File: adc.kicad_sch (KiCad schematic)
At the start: 37 parts, among them J5 Conn_01x03_Pin, J8 Conn_01x03_Pin, U21 LTC2299xUP

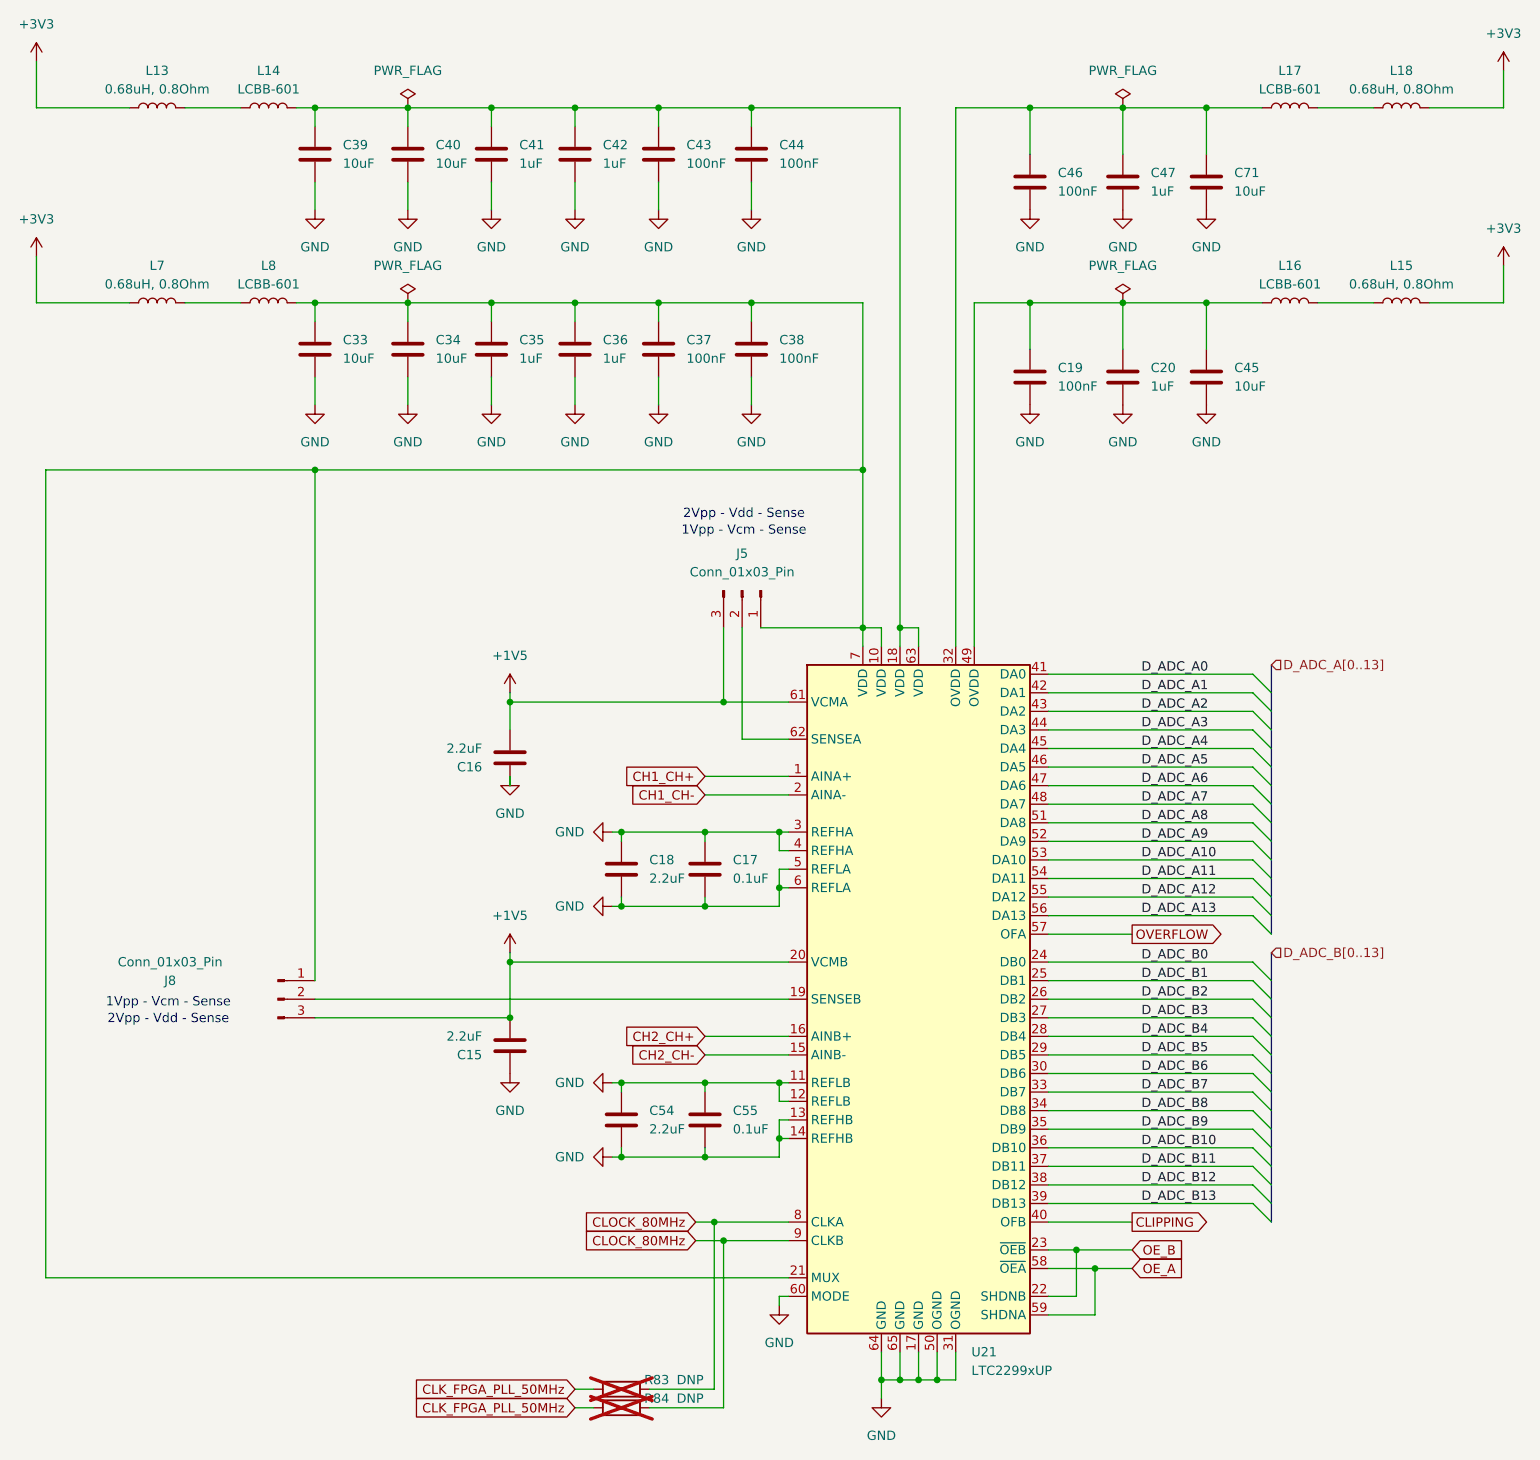
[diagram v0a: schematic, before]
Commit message: Add all footprints
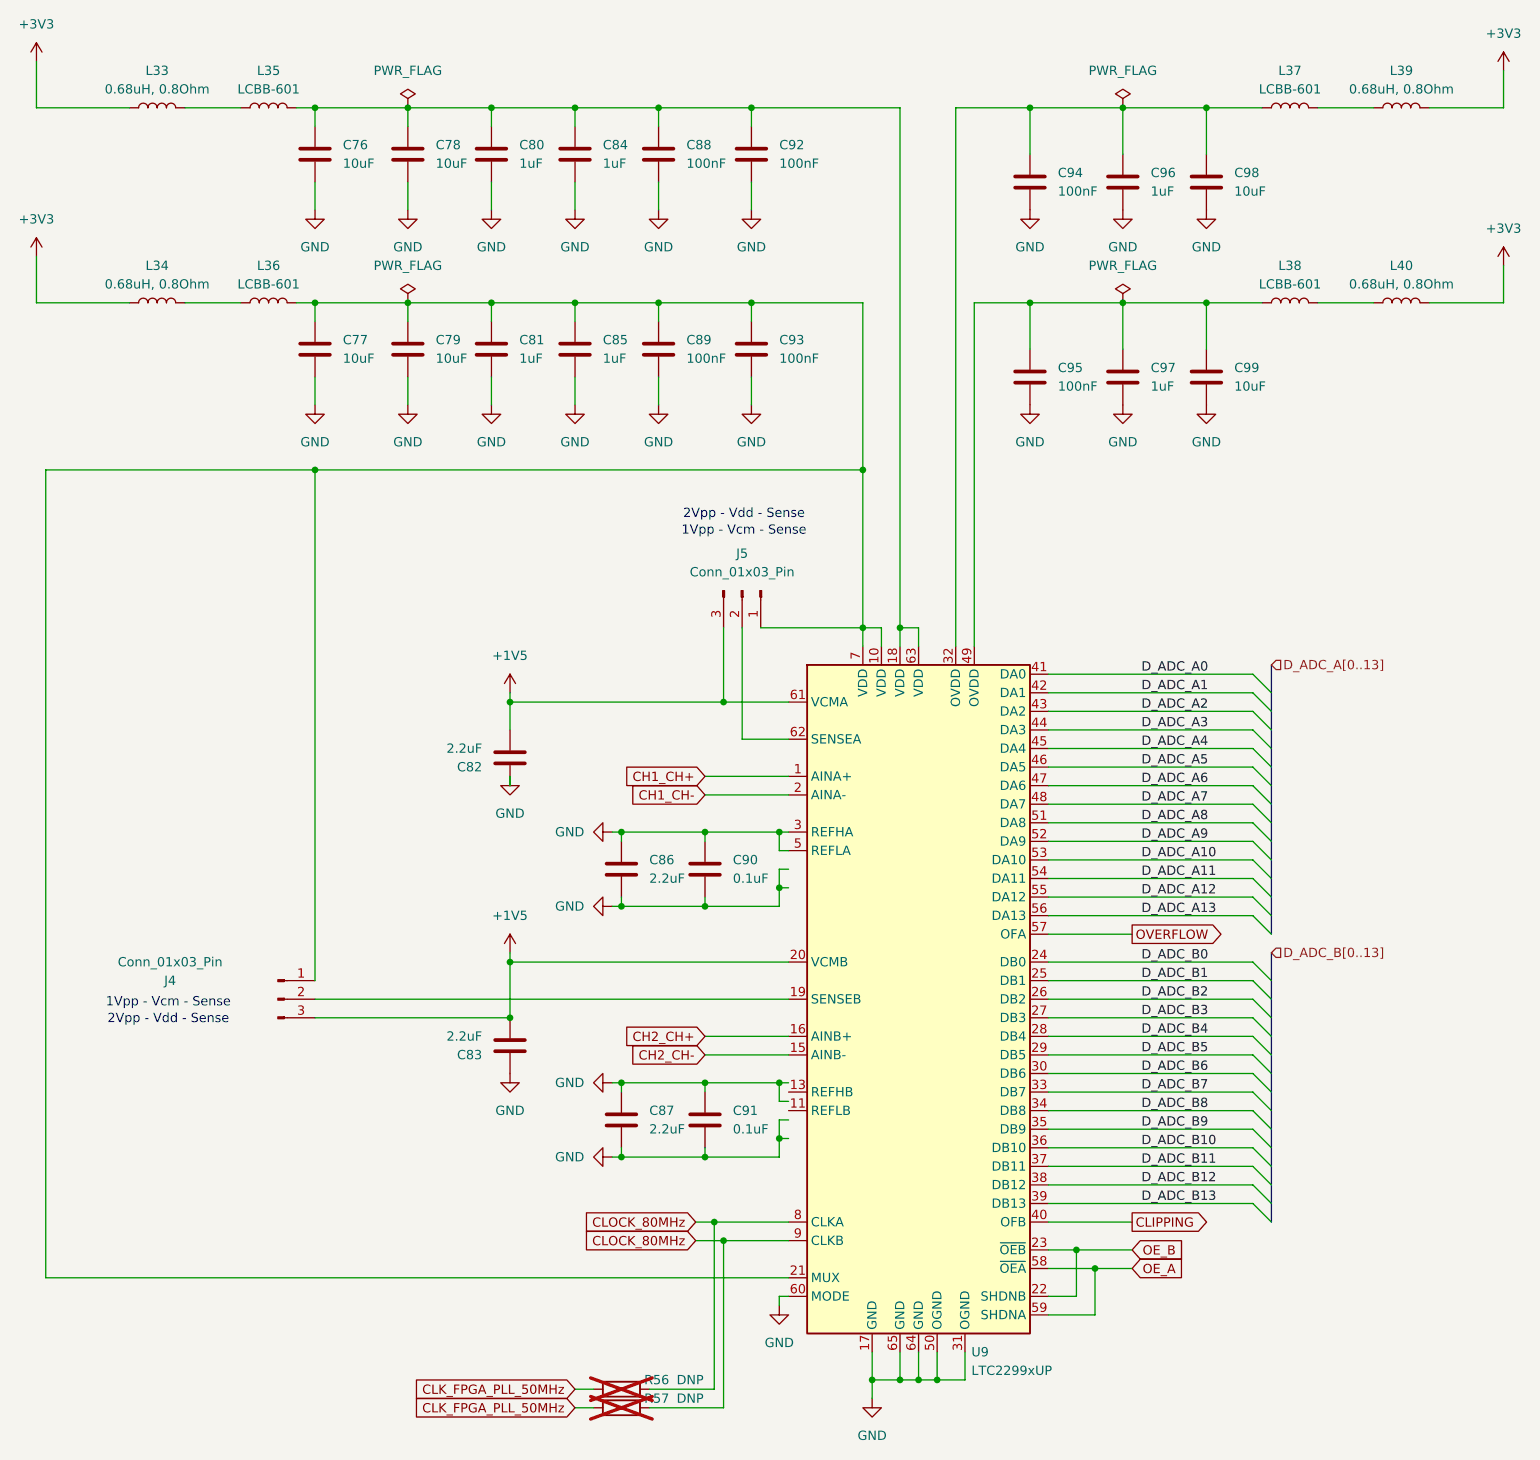
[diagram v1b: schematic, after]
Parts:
- J4: renamed from J8; footprint (none) -> TerminalBlock:TerminalBlock_MaiXu_MX126-5.0-03P_1x03_P5.00mm
- J5: footprint (none) -> TerminalBlock:TerminalBlock_MaiXu_MX126-5.0-03P_1x03_P5.00mm
- L33: renamed from L13; footprint (none) -> Inductor_SMD:L_0805_2012Metric
- L34: renamed from L7; footprint (none) -> Inductor_SMD:L_0805_2012Metric
- L35: renamed from L14; footprint (none) -> Inductor_SMD:L_0805_2012Metric
- L36: renamed from L8; footprint (none) -> Inductor_SMD:L_0805_2012Metric
- L37: renamed from L17; footprint (none) -> Inductor_SMD:L_0805_2012Metric
- L38: renamed from L16; footprint (none) -> Inductor_SMD:L_0805_2012Metric
- L39: renamed from L18; footprint (none) -> Inductor_SMD:L_0805_2012Metric
- L40: renamed from L15; footprint (none) -> Inductor_SMD:L_0805_2012Metric
- renumbered C39 to C76, C33 to C77, C40 to C78, C34 to C79, C41 to C80, C35 to C81, C16 to C82, C15 to C83, C42 to C84, C36 to C85, C18 to C86, C54 to C87, C43 to C88, C37 to C89, C17 to C90, C55 to C91, C44 to C92, C38 to C93, C46 to C94, C19 to C95, C47 to C96, C20 to C97, C71 to C98, C45 to C99, R83 to R56, R84 to R57, U21 to U9
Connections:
- net GND: no longer U9.11 (REFLB), U9.12 (REFLB), U9.13 (REFHB), U9.14 (REFHB)
- new net: U9.11 (REFLB), U9.12 (REFLB)
- new net: U9.13 (REFHB), U9.14 (REFHB)
